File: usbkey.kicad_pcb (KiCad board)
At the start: 2 copper layers, 13 x 11 mm, 16 parts, among them P1 USART0, P2 DEBUG, P3 USB_B, U1 EFM32HG309

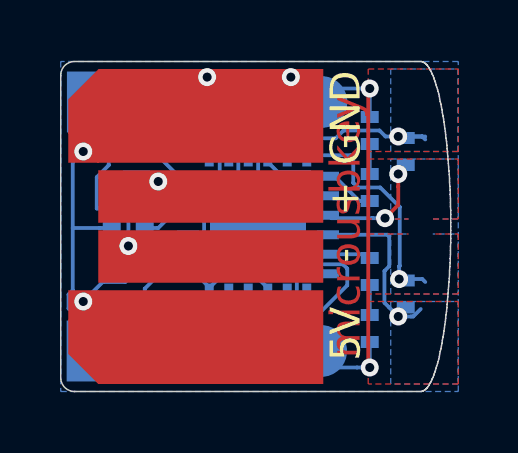
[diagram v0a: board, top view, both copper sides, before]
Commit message: Lots of small fixes.
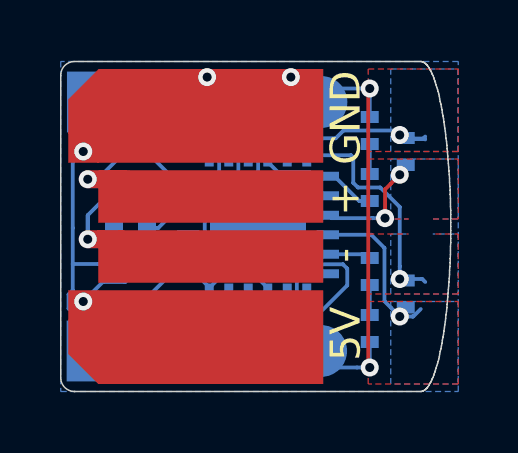
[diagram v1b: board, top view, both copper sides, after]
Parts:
- moved R3 0.45 mm to (19.5, 22.3)
- moved R4 0.45 mm to (19.5, 21.0)
- moved C1 0.07 mm to (19.3, 25.9)
- moved C2 0.07 mm to (19.3, 23.6)
- moved C3 0.07 mm to (19.3, 24.8)
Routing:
- net GND: track 41.2 -> 48.5 mm
- net /USB_D-: track 4.97 -> 7.43 mm
- net /RUSB_D-: track 1.99 -> 1.37 mm
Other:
- net class Default: clearance 0.127 -> 0.1016
- rule trace_clearance: 0.127 -> 0.1016
- board text removed: "microusbkey"
